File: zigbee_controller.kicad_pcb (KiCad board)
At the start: 2 copper layers, 55.5 x 62.9 mm, 74 parts, among them J1 KF635, J10 TerminalBlock_KF301-5.0, J11 TerminalBlock_KF301-5.0, J12 TerminalBlock_KF301-5.0, J13 TerminalBlock_KF301-5.0, J3 Conn_01x06, J4 Conn_01x07, J5 Conn_01x05, P1 USB_C_Receptacle_GCT_USB4105, Q2 IRLB3813, Q3 IRLB3813, Q4 IRLB3813, Q5 IRLB3813, SW2 EN, SW4 Boot, U1 TPS54560, U2 ESP32-C6-MINI-1, U4 TC4427, U5 TC4427, U6 RT9080, U9 CH224K

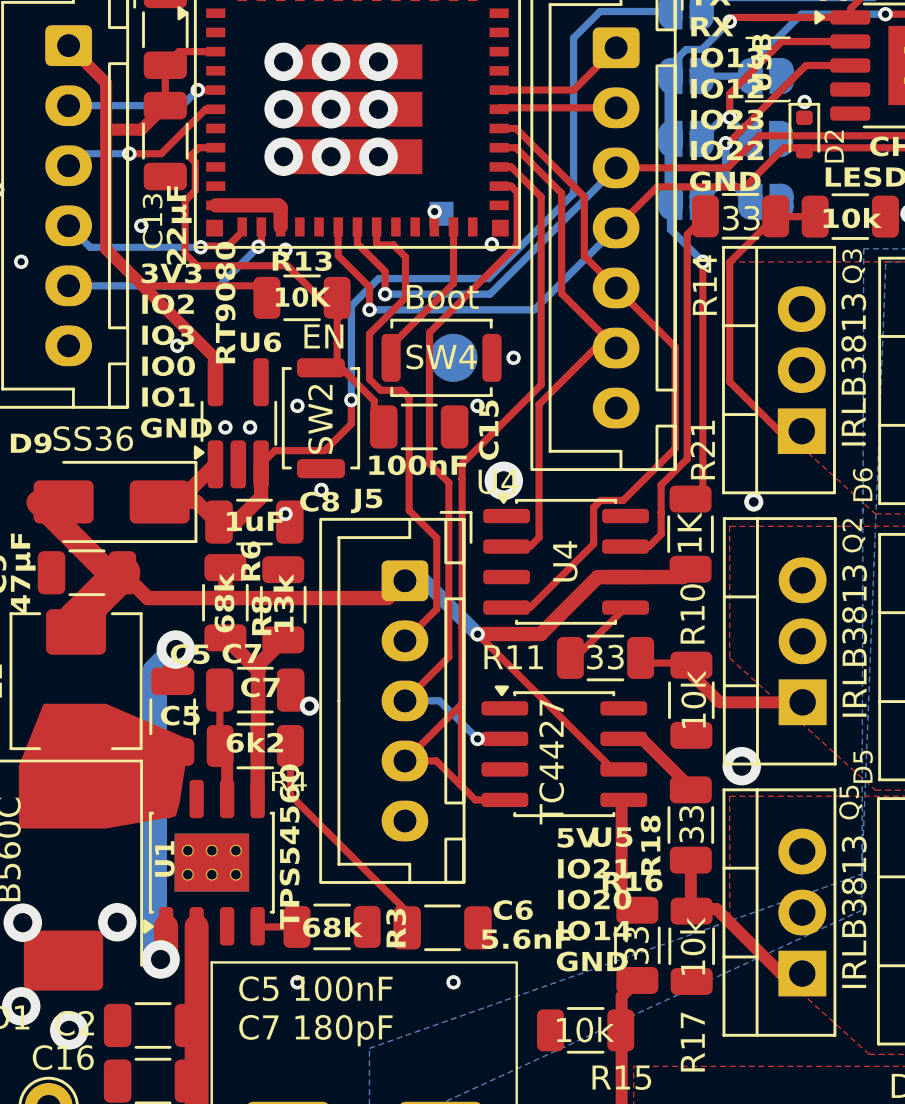
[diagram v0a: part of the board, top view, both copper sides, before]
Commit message: All errors and warning fixed
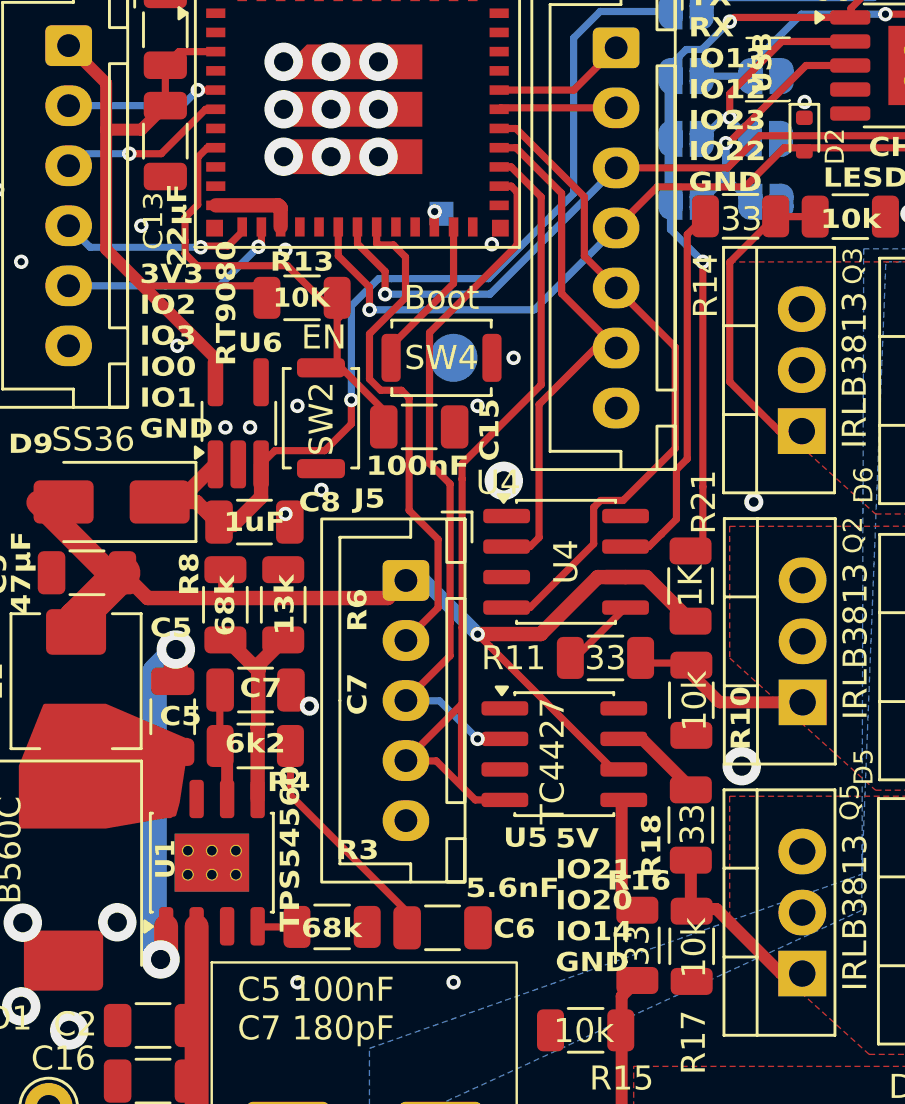
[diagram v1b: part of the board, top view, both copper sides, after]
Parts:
- moved R21 2.16 mm to (182.4, 101.5)
- moved R8 0.09 mm to (163.0, 102.2)
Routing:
- net /CH224k_Vdd: track 30.3 -> 32.4 mm
- net Net-(U2-EN): track 20.5 -> 19.5 mm
- net +5V: track 43.7 -> 44.4 mm
